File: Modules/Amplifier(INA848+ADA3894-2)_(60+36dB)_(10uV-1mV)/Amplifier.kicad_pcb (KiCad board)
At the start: 4 copper layers, 81.9 x 14.8 mm, 59 parts, among them J1 Conn_01x04, J2 Conn_01x01_Female, J3 Conn_01x03_Female, J4 Conn_01x02_Male, J5 Conn_01x01_Female, U1 TPS7A4901DGNR, U2 TPS7A3001DGNT, U3 ina848, U4 ADA4898-2, U5 ADA4898-2

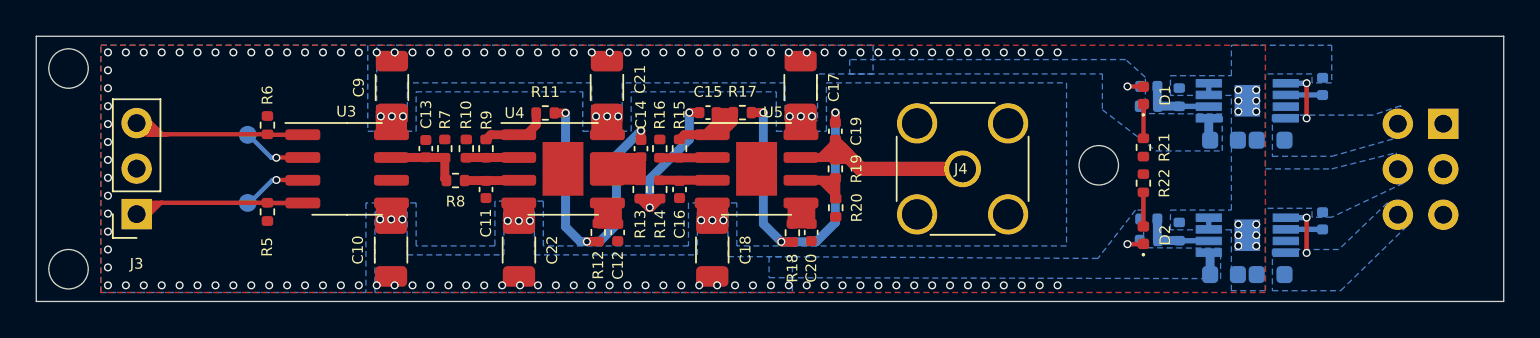
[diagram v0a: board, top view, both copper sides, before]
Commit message: update kicad editor version
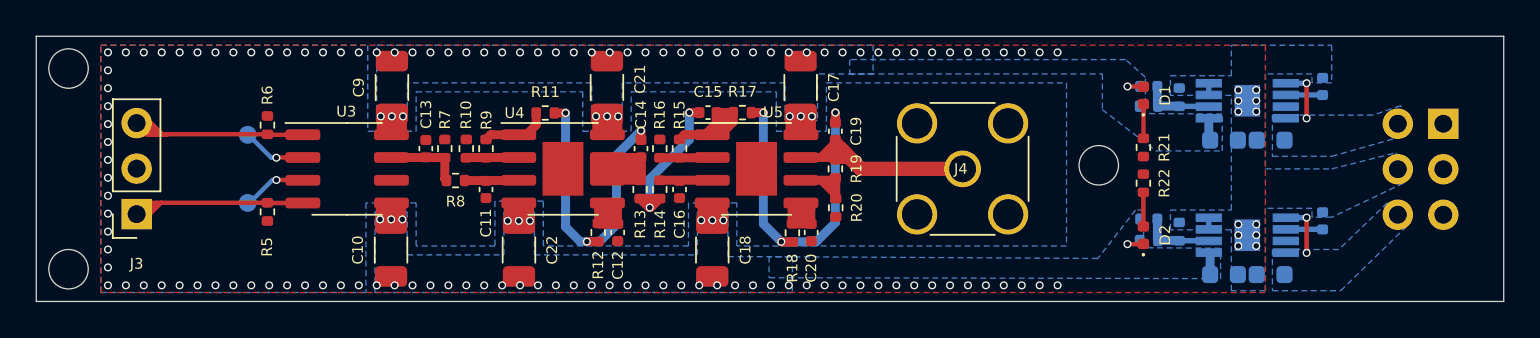
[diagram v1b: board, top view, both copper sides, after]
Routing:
- net AVEE: track 21.7 -> 14.0 mm
- net AVCC: track 21.7 -> 14.5 mm
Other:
- net class Default removed
